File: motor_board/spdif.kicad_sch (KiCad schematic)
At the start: 9 parts, among them IC1 TORX1950A_F_, U3 SN74AHC1G04DBVR

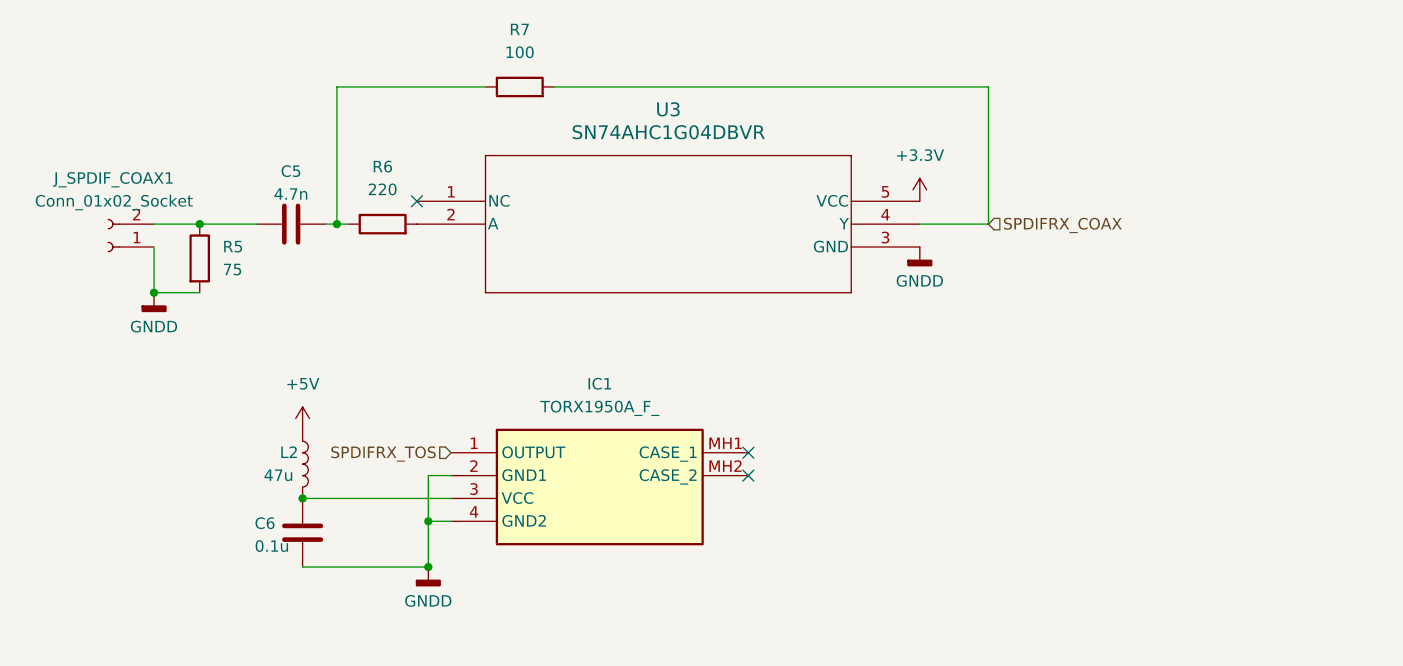
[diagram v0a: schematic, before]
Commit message: Began motor board layour
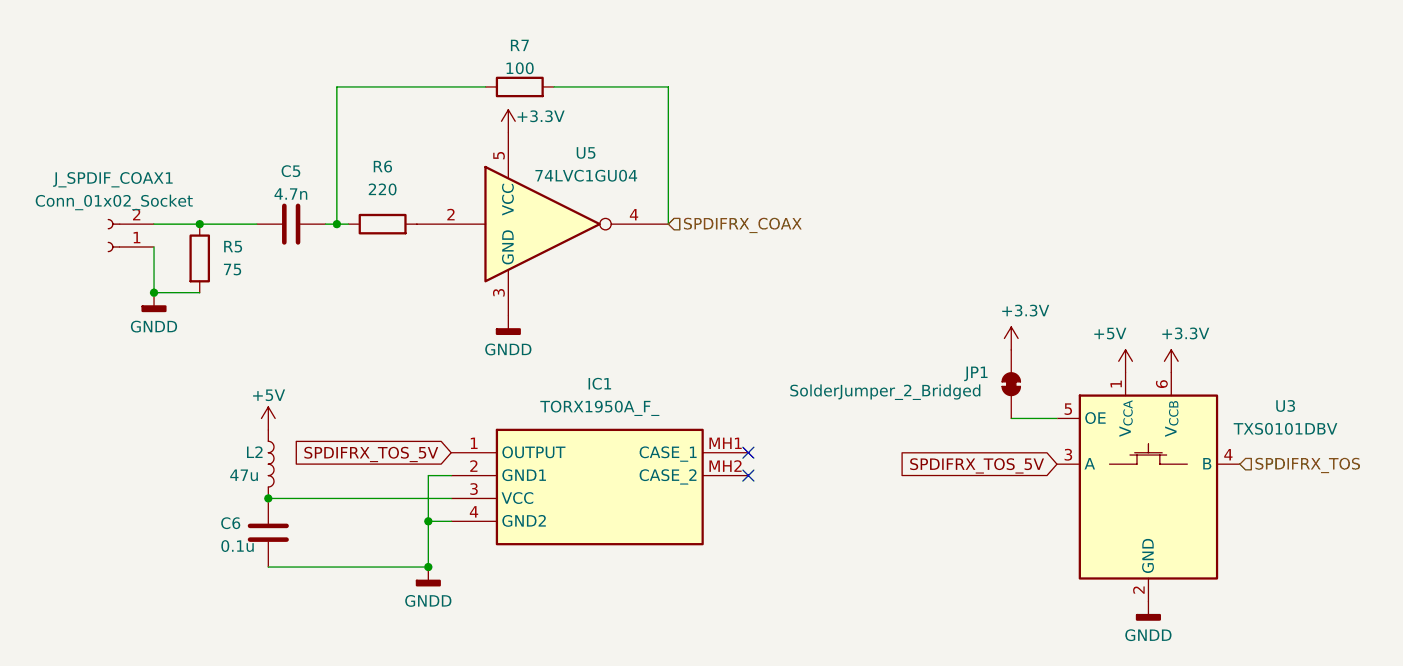
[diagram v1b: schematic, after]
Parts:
- removed U3: SN74AHC1G04DBVR, footprints_2:DBV5, symbol 2026-02-16_22-25-31:SN74AHC1G04DBVR
- added JP1: SolderJumper_2_Bridged, Jumper:SolderJumper-2_P1.3mm_Bridged_RoundedPad1.0x1.5mm, symbol Jumper:SolderJumper_2_Bridged
- added U3: TXS0101DBV, Package_TO_SOT_SMD:SOT-23-6, symbol Logic_LevelTranslator:TXS0101DBV
- added U5: 74LVC1GU04, Package_TO_SOT_SMD:SOT-23-5, symbol 74xGxx:74LVC1GU04
- C6: footprint Capacitor_SMD:C_0805_2012Metric_Pad1.18x1.45mm_HandSolder -> Capacitor_SMD:C_0603_1608Metric_Pad1.08x0.95mm_HandSolder
- L2: footprint (none) -> Inductor_SMD:L_Vishay_IHLP-4040
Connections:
- net +3.3V: now also JP1.2 (B), U3.6 (V_{CCB}), U5.5 (VCC)
- net +5V: now also U3.1 (V_{CCA})
- net GNDD: now also U3.2 (GND), U5.3 (GND)
- net SPDIFRX_COAX: now also U5.4
- net SPDIFRX_TOS: now also U3.4 (B); no longer IC1.1 (OUTPUT)
- net at R6.2: now also U5.2
- new net: JP1.1 (A), U3.5 (OE)
- new net SPDIFRX_TOS_5V: IC1.1 (OUTPUT), U3.3 (A)
- no-connect marks 3 -> 2
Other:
- moved on the sheet: C6, L2
